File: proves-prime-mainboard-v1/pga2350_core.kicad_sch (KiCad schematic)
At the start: 18 parts, among them SW1 KMR2, SW2 KMR2, SW4 SW_SPDT

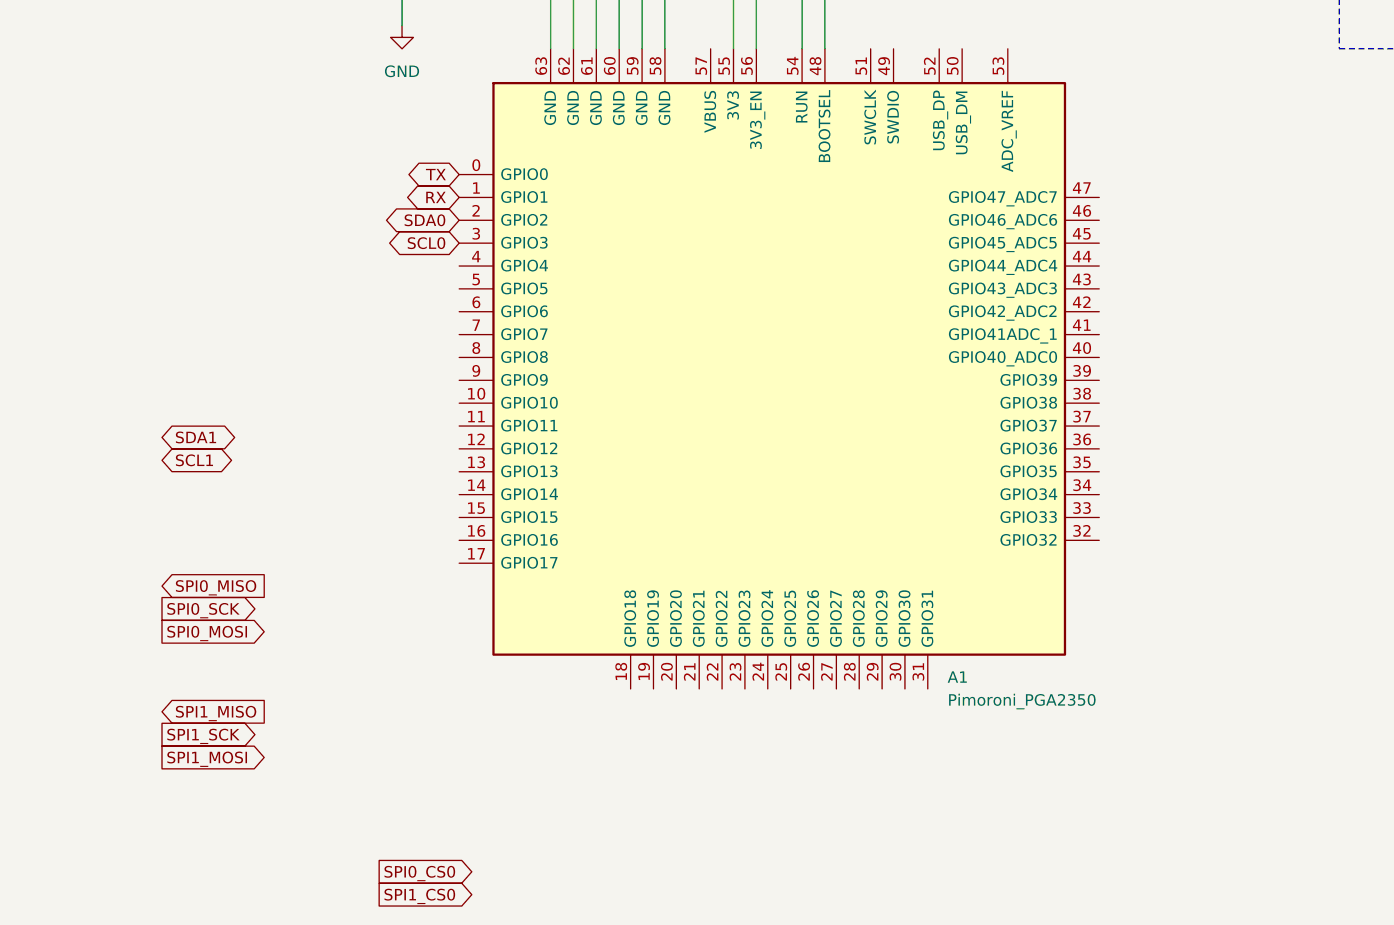
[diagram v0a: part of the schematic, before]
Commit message: DSAFASDFASDF
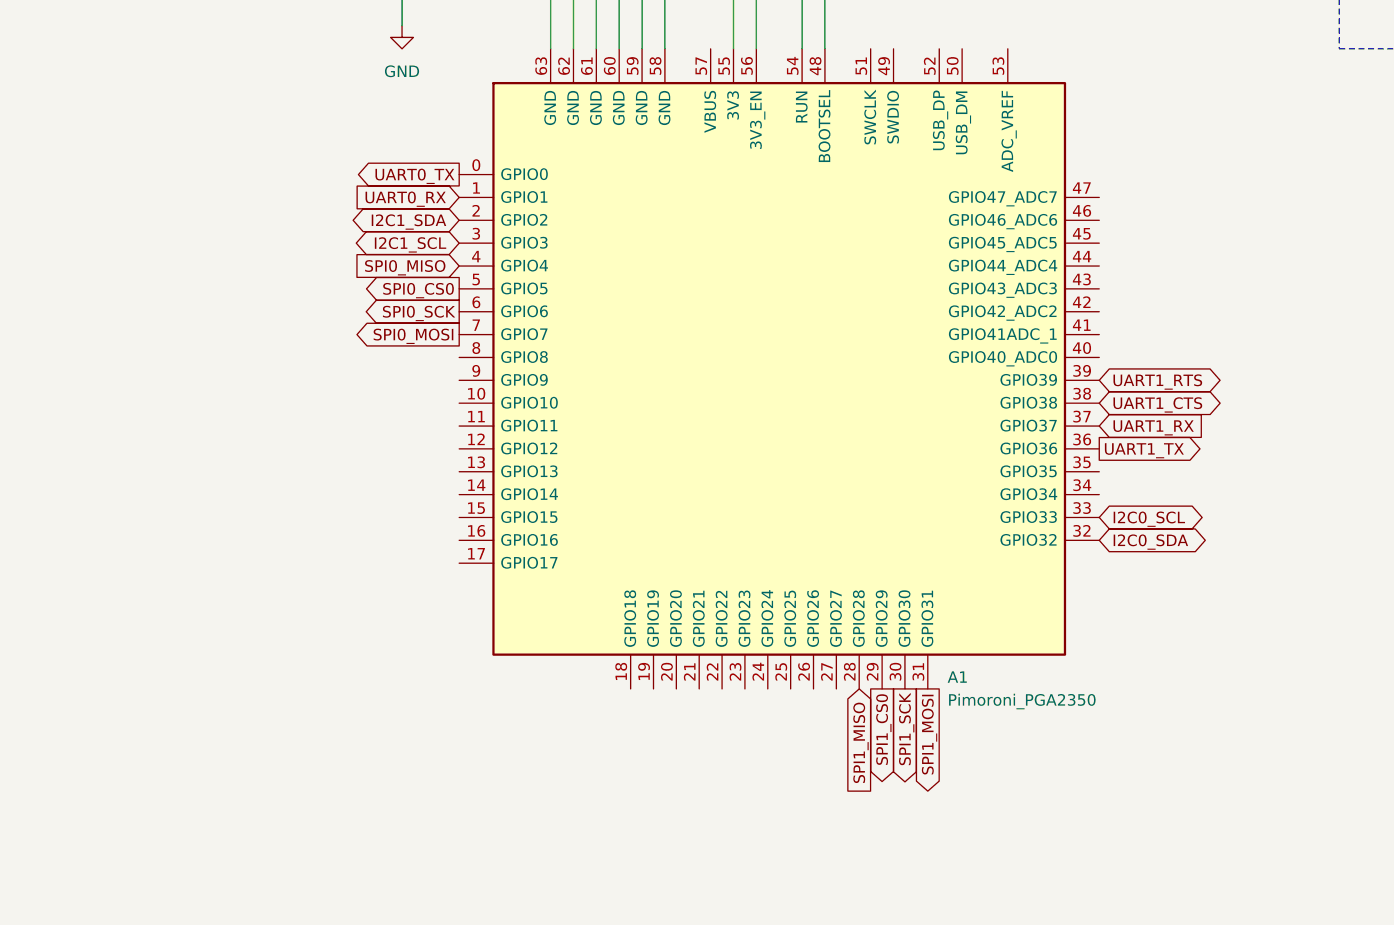
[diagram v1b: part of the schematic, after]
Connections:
- net RX: no longer A1.1 (GPIO1)
- net SPI0_CS0: now also A1.5 (GPIO5)
- net SPI0_MISO: now also A1.4 (GPIO4)
- net SPI0_MOSI: now also A1.7 (GPIO7)
- net SPI0_SCK: now also A1.6 (GPIO6)
- net SPI1_CS0: now also A1.29 (GPIO29)
- net SPI1_MISO: now also A1.28 (GPIO28)
- net SPI1_MOSI: now also A1.31 (GPIO31)
- net SPI1_SCK: now also A1.30 (GPIO30)
- net TX: no longer A1.0 (GPIO0)
- net I2C0_SDA: now reaches A1.32 (GPIO32)
- net I2C0_SCL: now reaches A1.33 (GPIO33)
- net UART1_TX: now reaches A1.36 (GPIO36)
- net UART1_RX: now reaches A1.37 (GPIO37)
- net UART1_CTS: now reaches A1.38 (GPIO38)
- net UART1_RTS: now reaches A1.39 (GPIO39)
- net SCL0 renamed I2C1_SCL
- net SDA0 renamed I2C1_SDA
- new net UART0_RX: A1.1 (GPIO1)
- new net UART0_TX: A1.0 (GPIO0)
